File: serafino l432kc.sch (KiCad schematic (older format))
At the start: 31 parts, among them J1 USB_B_Micro, J2 Conn_01x14, J3 Conn_01x14, Q1 SI3401A-TP, SW1 SW_Push, SW2 SW_Push, U1 AP2112K-3.3, U2 USBLC6-2SC6, U3 STM32L432KCUx, Y1 32.768K

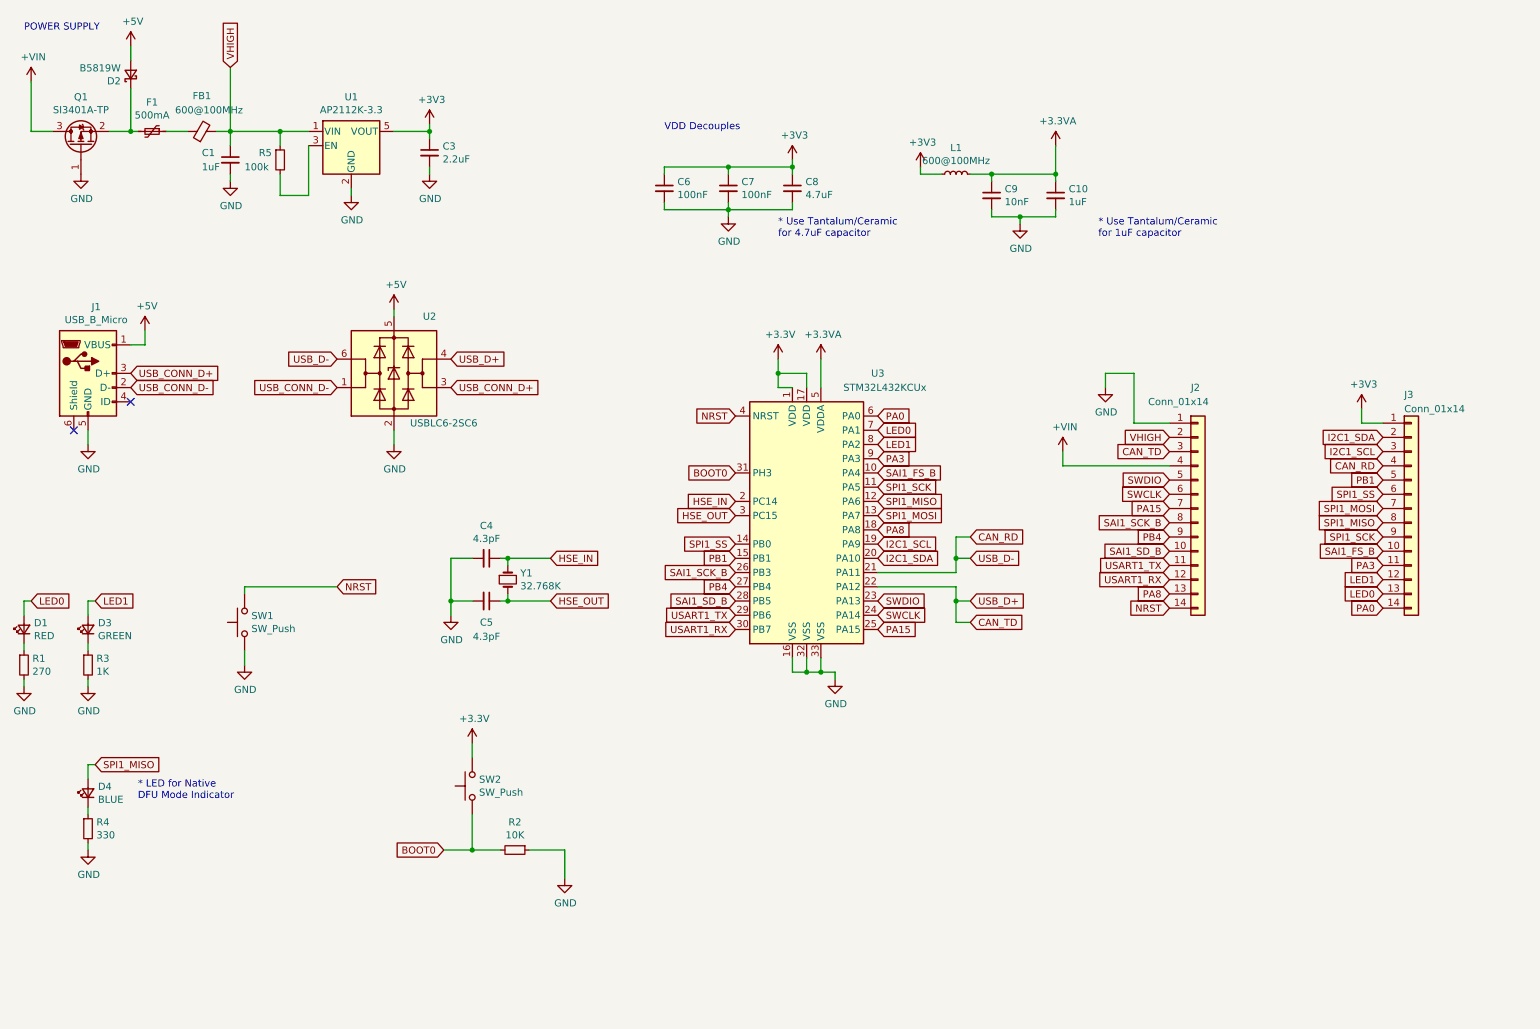
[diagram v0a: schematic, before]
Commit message: Led Specs
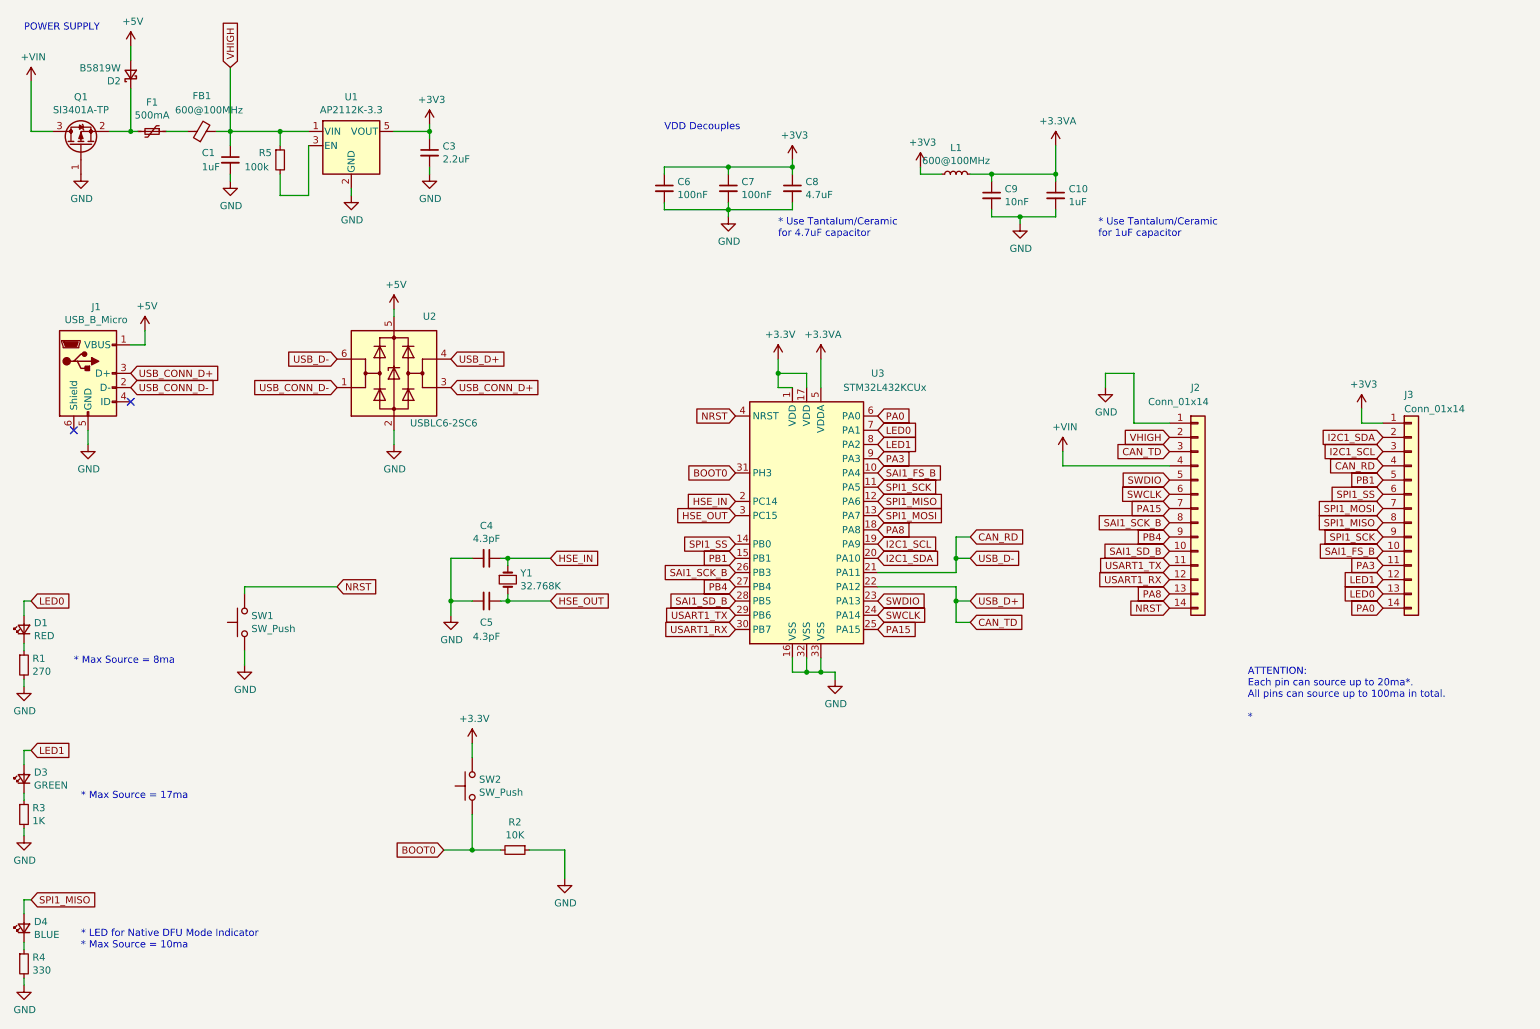
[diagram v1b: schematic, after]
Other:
- note added: "* LED for Native DFU Mode Indicator\n* Max Source = 10ma"
- note added: "* Max Source = 17ma"
- note added: "* Max Source = 8ma"
- note added: "ATTENTION:\nEach pin can source up to 20ma*. \nAll pins can source up to 100ma in total.\n\n*"
- note removed: "* LED for Native \nDFU Mode Indicator"
- moved on the sheet: D3, D4, R3, R4
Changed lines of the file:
@@
 encoding utf-8
 Sheet 1 1
-Title ""
-Date ""
-Rev ""
-Comp ""
-Comment1 ""
+Title "Seraph L432KC"
+Date "2021-02-04"
+Rev "1.0"
+Comp "MATERIAM"
+Comment1 "Breakout board for STM32L432KC"
 Comment2 ""
 Comment3 ""
@@
 L Device:R_Small R3
 U 1 1 5FD4E68B
-P 1150 5150
-F 0 "R3" H 1209 5196 50  0000 L CNN
-F 1 "1K" H 1209 5105 50  0000 L CNN
-F 2 "Resistor_SMD:R_0603_1608Metric" H 1150 5150 50  0001 C CNN
-F 3 "~" H 1150 5150 50  0001 C CNN
-F 4 "RC0603FR-071KL" H 1150 5150 50  0001 C CNN "Part No."
-	1    1150 5150
+P 700 6200
+F 0 "R3" H 759 6246 50  0000 L CNN
+F 1 "1K" H 759 6155 50  0000 L CNN
+F 2 "Resistor_SMD:R_0603_1608Metric" H 700 6200 50  0001 C CNN
+F 3 "~" H 700 6200 50  0001 C CNN
+F 4 "RC0603FR-071KL" H 700 6200 50  0001 C CNN "Part No."
+	1    700  6200
 	1    0    0    -1
 $EndComp
@@
 L Device:LED_Small D3
 U 1 1 5FD4E887
-P 1150 4900
-F 0 "D3" V 1196 4830 50  0000 R CNN
-F 1 "GREEN" V 1105 4830 50  0000 R CNN
-F 2 "LED_SMD:LED_0603_1608Metric" V 1150 4900 50  0001 C CNN
-F 3 "~" V 1150 4900 50  0001 C CNN
-F 4 "155060GS75300" H 1150 4900 50  0001 C CNN "Part No."
-	1    1150 4900
+P 700 5950
+F 0 "D3" V 746 5880 50  0000 R CNN
+F 1 "GREEN" V 655 5880 50  0000 R CNN
+F 2 "LED_SMD:LED_0603_1608Metric" V 700 5950 50  0001 C CNN
+F 3 "~" V 700 5950 50  0001 C CNN
+F 4 "155060GS75300" H 700 5950 50  0001 C CNN "Part No."
+	1    700  5950
 	0    -1   -1   0
 $EndComp
@@
 L power:GND #PWR0106
 U 1 1 5FD4EB85
-P 1150 5300
-F 0 "#PWR0106" H 1150 5050 50  0001 C CNN
-F 1 "GND" H 1155 5127 50  0000 C CNN
-F 2 "" H 1150 5300 50  0001 C CNN
-F 3 "" H 1150 5300 50  0001 C CNN
-	1    1150 5300
+P 700 6350
+F 0 "#PWR0106" H 700 6100 50  0001 C CNN
+F 1 "GND" H 705 6177 50  0000 C CNN
+F 2 "" H 700 6350 50  0001 C CNN
+F 3 "" H 700 6350 50  0001 C CNN
+	1    700  6350
 	1    0    0    -1
 $EndComp
@@
 L Device:R_Small R4
 U 1 1 5FD4ED72
-P 1150 6300
-F 0 "R4" H 1209 6346 50  0000 L CNN
-F 1 "330" H 1209 6255 50  0000 L CNN
-F 2 "Resistor_SMD:R_0603_1608Metric" H 1150 6300 50  0001 C CNN
-F 3 "~" H 1150 6300 50  0001 C CNN
-F 4 "RC0603FR-071KL" H 1150 6300 50  0001 C CNN "Part No."
-	1    1150 6300
+P 700 7250
+F 0 "R4" H 759 7296 50  0000 L CNN
+F 1 "330" H 759 7205 50  0000 L CNN
+F 2 "Resistor_SMD:R_0603_1608Metric" H 700 7250 50  0001 C CNN
+F 3 "~" H 700 7250 50  0001 C CNN
+F 4 "RC0603FR-071KL" H 700 7250 50  0001 C CNN "Part No."
+	1    700  7250
 	1    0    0    -1
 $EndComp
@@
 L power:GND #PWR0108
 U 1 1 5FD4F1E4
-P 1150 6450
-F 0 "#PWR0108" H 1150 6200 50  0001 C CNN
-F 1 "GND" H 1155 6277 50  0000 C CNN
-F 2 "" H 1150 6450 50  0001 C CNN
-F 3 "" H 1150 6450 50  0001 C CNN
-	1    1150 6450
+P 700 7400
+F 0 "#PWR0108" H 700 7150 50  0001 C CNN
+F 1 "GND" H 705 7227 50  0000 C CNN
+F 2 "" H 700 7400 50  0001 C CNN
+F 3 "" H 700 7400 50  0001 C CNN
+	1    700  7400
 	1    0    0    -1
 $EndComp
@@
 L Device:LED_Small D4
 U 1 1 5FD4F3F3
-P 1150 6050
-F 0 "D4" V 1196 5980 50  0000 R CNN
-F 1 "BLUE" V 1105 5980 50  0000 R CNN
-F 2 "LED_SMD:LED_0603_1608Metric" V 1150 6050 50  0001 C CNN
-F 3 "~" V 1150 6050 50  0001 C CNN
-F 4 "155060BS75300" H 1150 6050 50  0001 C CNN "Part No."
-	1    1150 6050
+P 700 7000
+F 0 "D4" V 746 6930 50  0000 R CNN
+F 1 "BLUE" V 655 6930 50  0000 R CNN
+F 2 "LED_SMD:LED_0603_1608Metric" V 700 7000 50  0001 C CNN
+F 3 "~" V 700 7000 50  0001 C CNN
+F 4 "155060BS75300" H 700 7000 50  0001 C CNN "Part No."
+	1    700  7000
 	0    -1   -1   0
 $EndComp
 Wire Wire Line
-	1150 5000 1150 5050
-Wire Wire Line
-	1150 6150 1150 6200
-Wire Wire Line
-	1150 5250 1150 5300
-Wire Wire Line
-	1150 6400 1150 6450
-Text GLabel 1200 4700 2    50   Input ~ 0
+	700  6050 700  6100
+Wire Wire Line
+	700  7100 700  7150
+Wire Wire Line
+	700  6300 700  6350
+Wire Wire Line
+	700  7350 700  7400
+Text GLabel 750  5750 2    50   Input ~ 0
 LED1
 Wire Wire Line
-	1200 4700 1150 4700
-Wire Wire Line
-	1150 4700 1150 4800
-Wire Wire Line
-	1200 5850 1150 5850
-Wire Wire Line
-	1150 5850 1150 5950
+	750  5750 700  5750
+Wire Wire Line
+	700  5750 700  5850
+Wire Wire Line
+	750  6800 700  6800
+Wire Wire Line
+	700  6800 700  6900
 Connection ~ 1450 1400
 Wire Wire Line
@@
 Wire Wire Line
 	3850 6450 4050 6450
-Text GLabel 1200 5850 2    50   Input ~ 0
+Text GLabel 750  6800 2    50   Input ~ 0
 SPI1_MISO
-Text Notes 1500 6100 0    50   ~ 0
-* LED for Native \nDFU Mode Indicator
+Text Notes 1100 7150 0    50   ~ 0
+* LED for Native DFU Mode Indicator\n* Max Source = 10ma
 Text GLabel 8750 4250 0    50   Input ~ 0
 PB4
@@
 	7250 4850 7250 4700
 Connection ~ 7250 4700
+Text Notes 1100 6100 0    50   ~ 0
+* Max Source = 17ma
+Text Notes 1050 5150 0    50   ~ 0
+* Max Source = 8ma
+Text Notes 9300 5550 0    50   ~ 0
+ATTENTION:\nEach pin can source up to 20ma*. \nAll pins can source up to 100ma in total.\n\n*
 $EndSCHEMATC
